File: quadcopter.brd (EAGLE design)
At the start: 203.5 x 203.5 mm, 73 parts, among them J1 AVR_SPI_PRG_6NS, U3 ATMEGA128RFA1

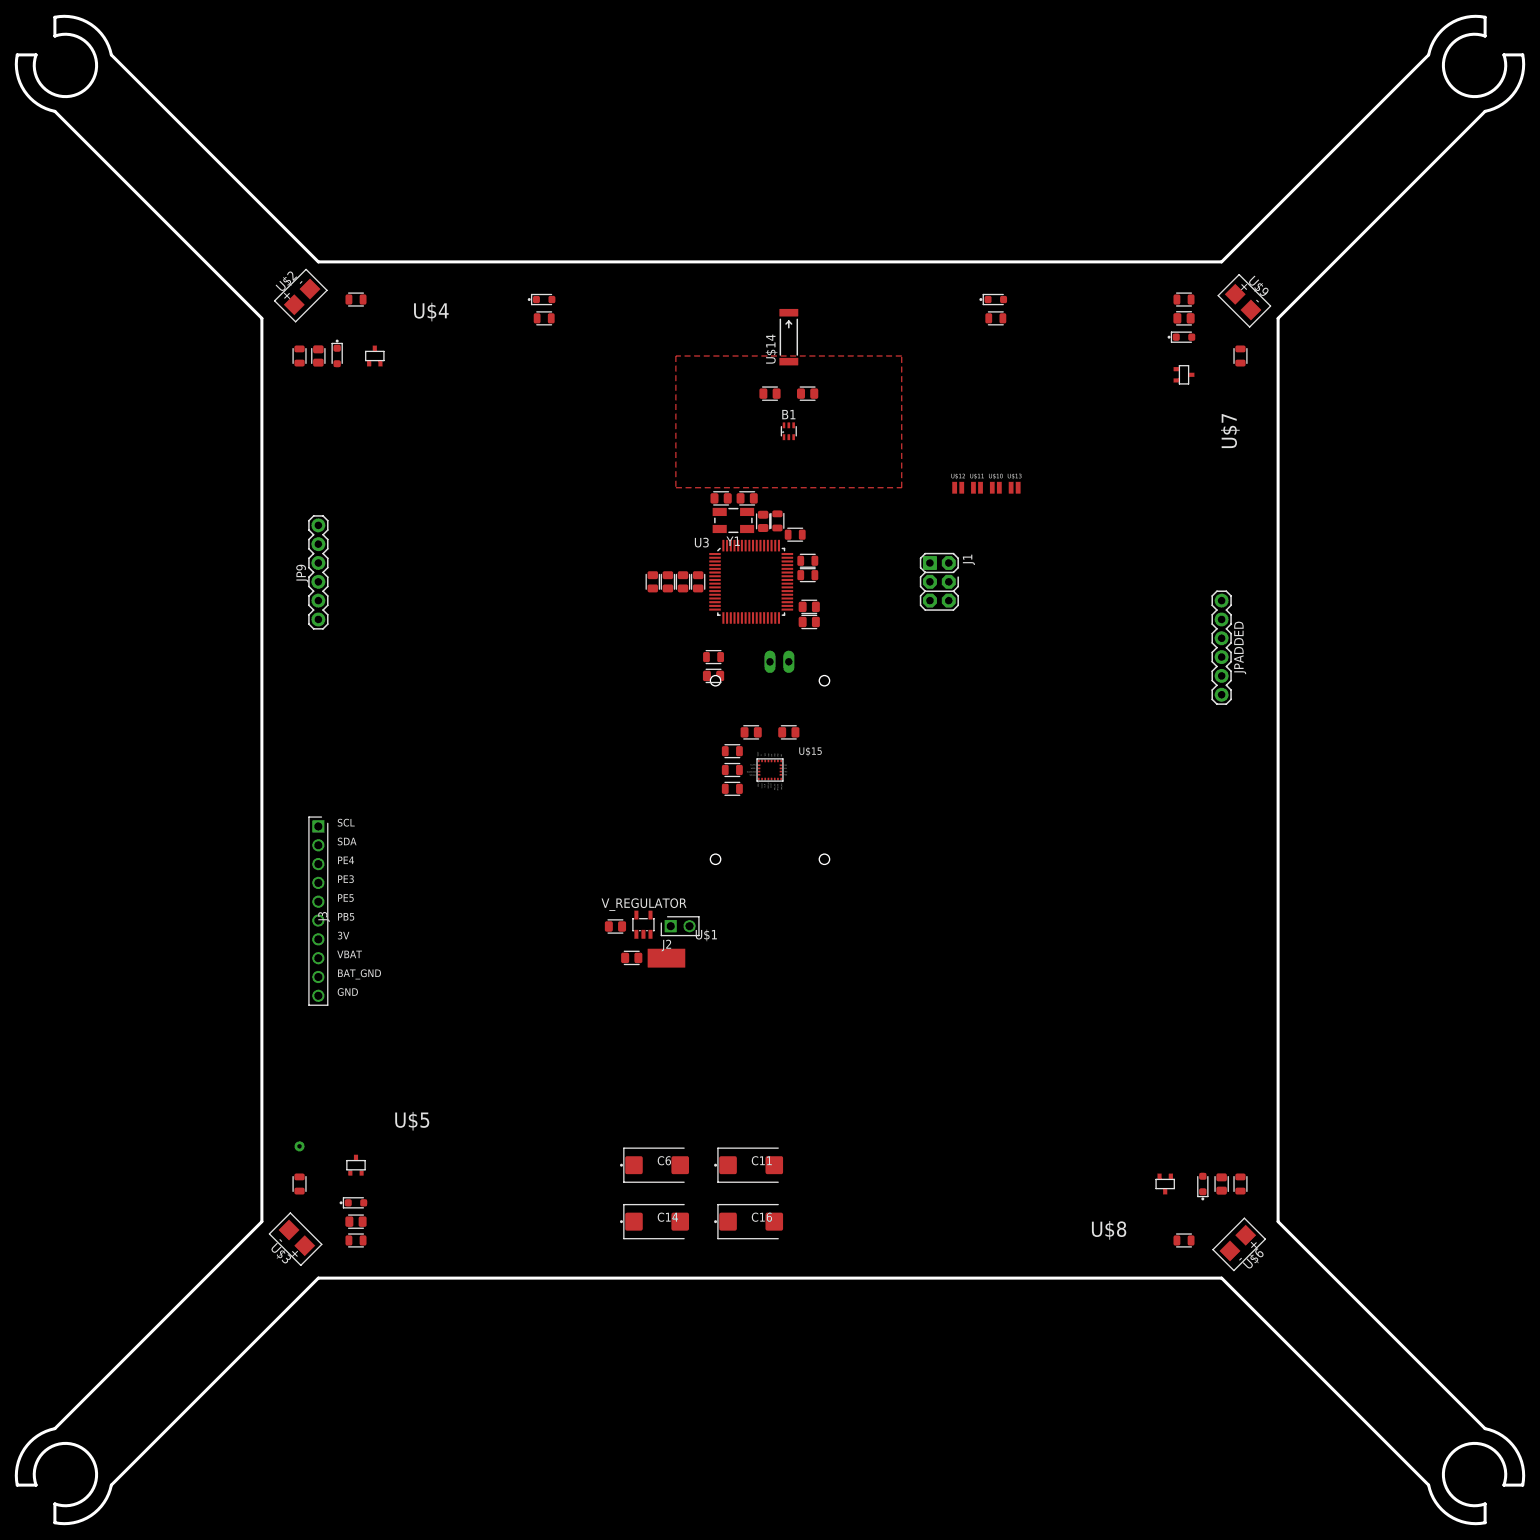
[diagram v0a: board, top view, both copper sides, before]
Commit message: almost done with board, have 3 airwires
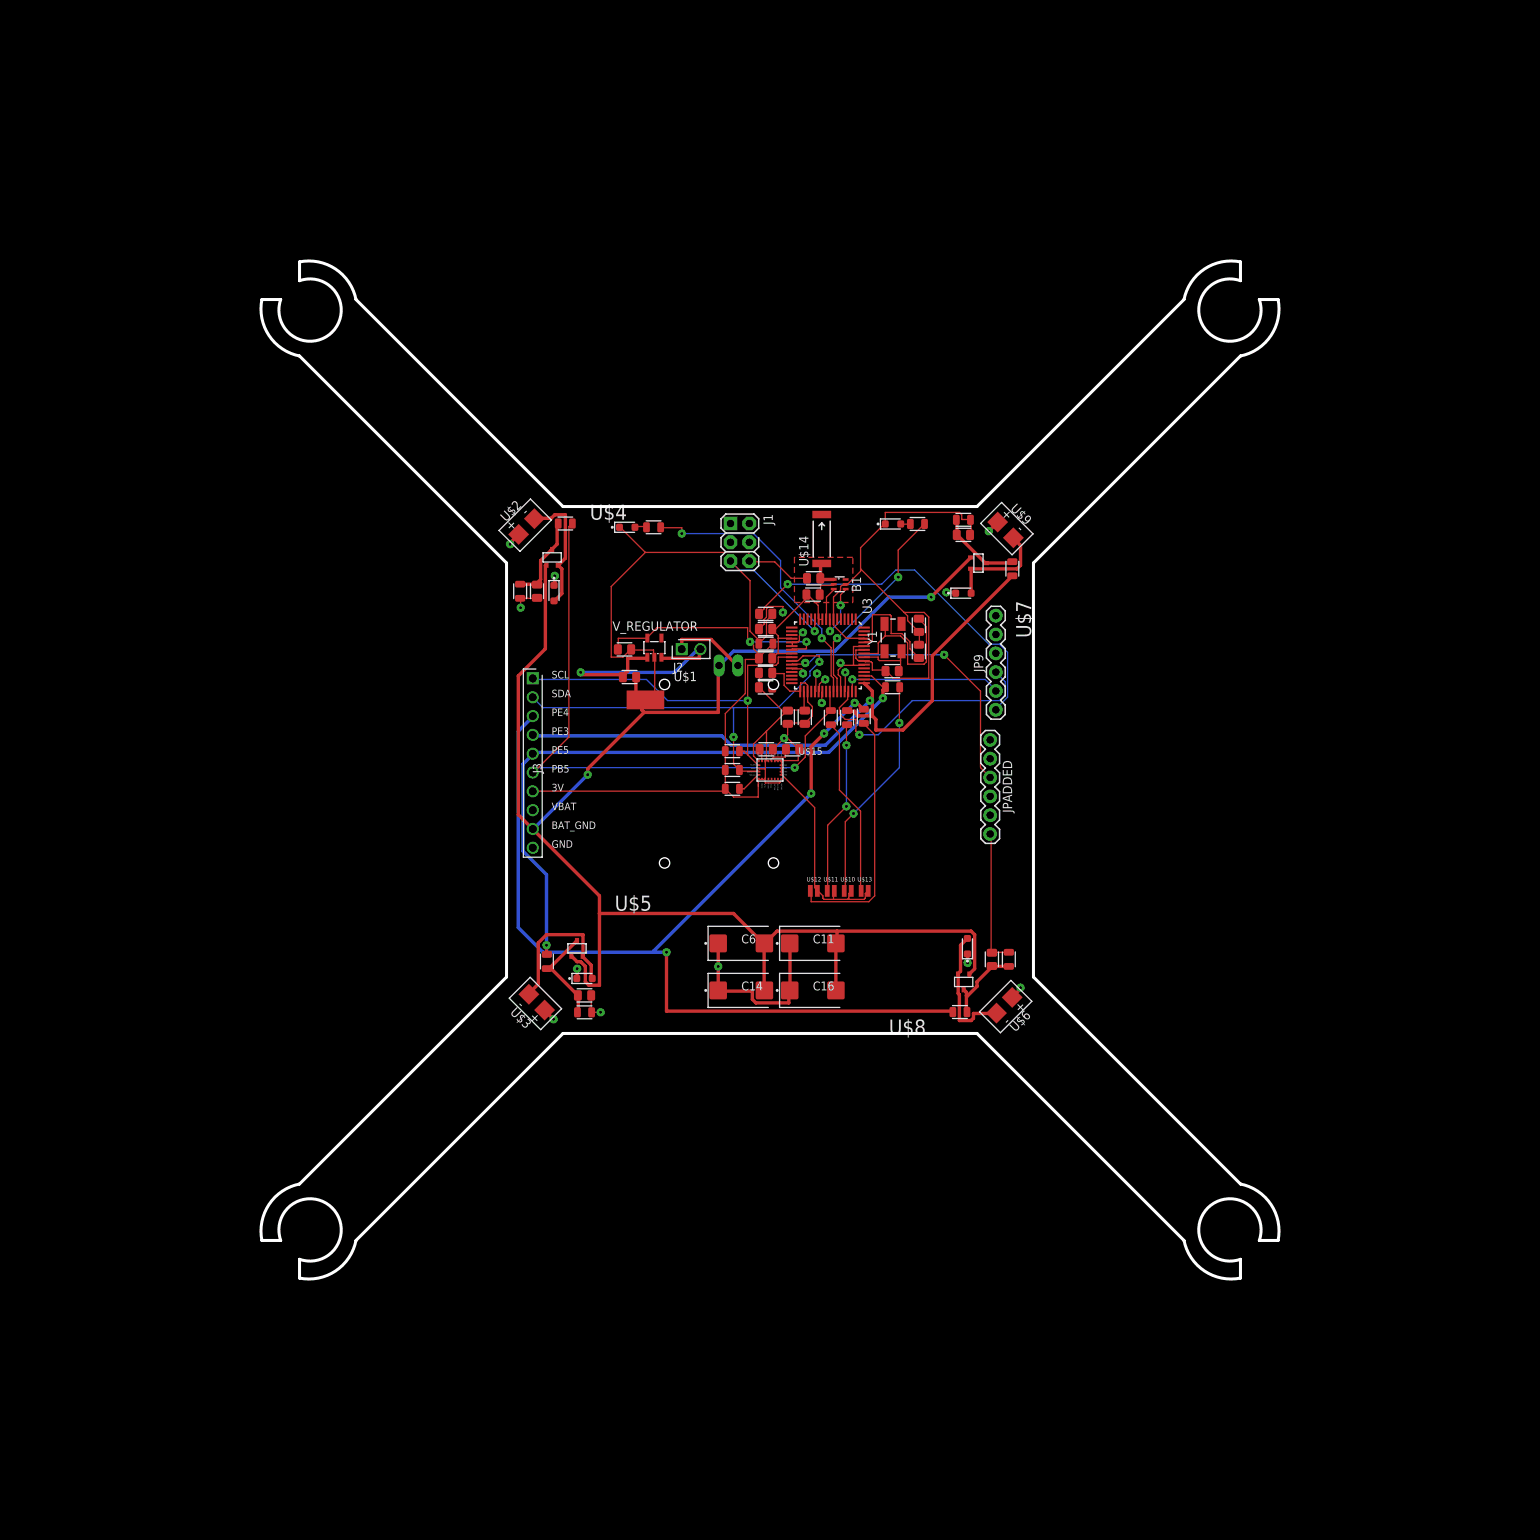
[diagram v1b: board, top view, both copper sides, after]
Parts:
- moved JP9 92.2 mm to (30.5, 8.13)
- moved U$13 58.1 mm to (12.8, -16.3)
- moved U$10 58.0 mm to (10.5, -16.3)
- moved U$11 57.9 mm to (8.21, -16.3)
- moved U$12 57.8 mm to (5.92, -16.3)
- moved D4 45.6 mm to (26.1, 23.9)
- moved U$3 45.4 mm to (-31.1, -31.7)
- moved D3 45.2 mm to (26.6, -23.8)
- moved U$6 45.0 mm to (32.0, -31.4)
- moved R2 44.9 mm to (-30.1, -25.9)
- moved U$9 44.4 mm to (31.4, 32.8)
- moved R5 43.6 mm to (-25.0, -32.7)
- moved R12 43.6 mm to (32.2, -25.6)
- moved R4 43.5 mm to (-33.7, 24.1)
- moved C13 43.4 mm to (-25.0, -30.4)
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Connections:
- net BAT_GND: now also BATT1.-, U$1.P$1; no longer U$1.P$2
- net GND: now also U$1.P$2; no longer BATT1.-, U$1.P$1
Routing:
- net GND: track 0.00 -> 242.8 mm, vias 0 -> 4
- net BAT_GND: track 0.00 -> 226.4 mm, vias 0 -> 2
- net PE4: track 0.00 -> 143.9 mm, vias 0 -> 4
- net 3V: track 0.00 -> 142.7 mm, vias 0 -> 3
- net PE3: track 0.00 -> 90.3 mm, vias 0 -> 1
- net PE5: track 0.00 -> 84.8 mm, vias 0 -> 2
- net VCC: track 0.00 -> 84.2 mm, vias 0 -> 10
- net PB5: track 0.00 -> 83.9 mm, vias 0 -> 1
- net SDA: track 0.00 -> 58.6 mm, vias 0 -> 2
- net SCL: track 0.00 -> 52.6 mm, vias 0 -> 1
- net N$21: track 0.00 -> 49.1 mm, vias 0 -> 1
- net RX1: track 0.00 -> 40.3 mm, vias 0 -> 2
- net PB6: track 0.00 -> 39.1 mm, vias 0 -> 2
- net RESET: track 0.00 -> 34.6 mm, vias 0 -> 1
- net N$9: track 0.00 -> 34.3 mm
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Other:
- board size 203.5 x 203.5 mm -> 137.4 x 137.4 mm
